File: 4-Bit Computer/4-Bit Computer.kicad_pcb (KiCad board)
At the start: 4 copper layers, 220.5 x 182.4 mm, 295 parts, among them J1 +12v, Q1 BC547, Q10 BC547, Q11 BC547, Q12 BC547, Q13 BC547, Q14 BC547, Q15 BC547, Q16 BC547, Q17 BC547, Q18 BC547, Q19 BC547, Q2 BC547, Q20 BC547, Q21 BC547, Q22 BC547, Q23 BC547, Q24 BC547, Q25 BC547, Q26 BC547, Q27 BC547, Q28 BC547, Q29 BC547, Q3 BC547, Q30 BC547, Q31 BC547, Q32 BC547, Q33 BC547, Q34 BC547, Q35 BC547, Q36 BC547, Q37 BC547, Q38 BC547, Q39 BC547, Q4 BC547, Q40 BC547, Q41 BC547, Q42 BC547, Q43 BC547, Q44 BC547, Q45 BC547, Q46 BC547, Q47 BC547, Q48 BC547, Q49 BC547, Q5 BC547, Q50 BC547, Q51 BC547, Q52 BC547, Q53 BC547, Q54 BC547, Q55 BC547, Q56 BC547, Q57 BC547, Q58 BC547, Q59 BC547, Q6 BC547, Q60 BC547, Q61 BC547, Q62 BC547, Q63 BC547, Q64 BC547, Q65 BC547, Q66 BC547, Q67 BC547, Q68 BC547, Q69 BC547, Q7 BC547, Q70 BC547, Q71 BC547, Q72 BC547, Q73 BC547, Q74 BC547, Q75 BC547, Q76 BC547, Q77 BC547, Q78 BC547, Q79 BC547, Q8 BC547, Q80 BC547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

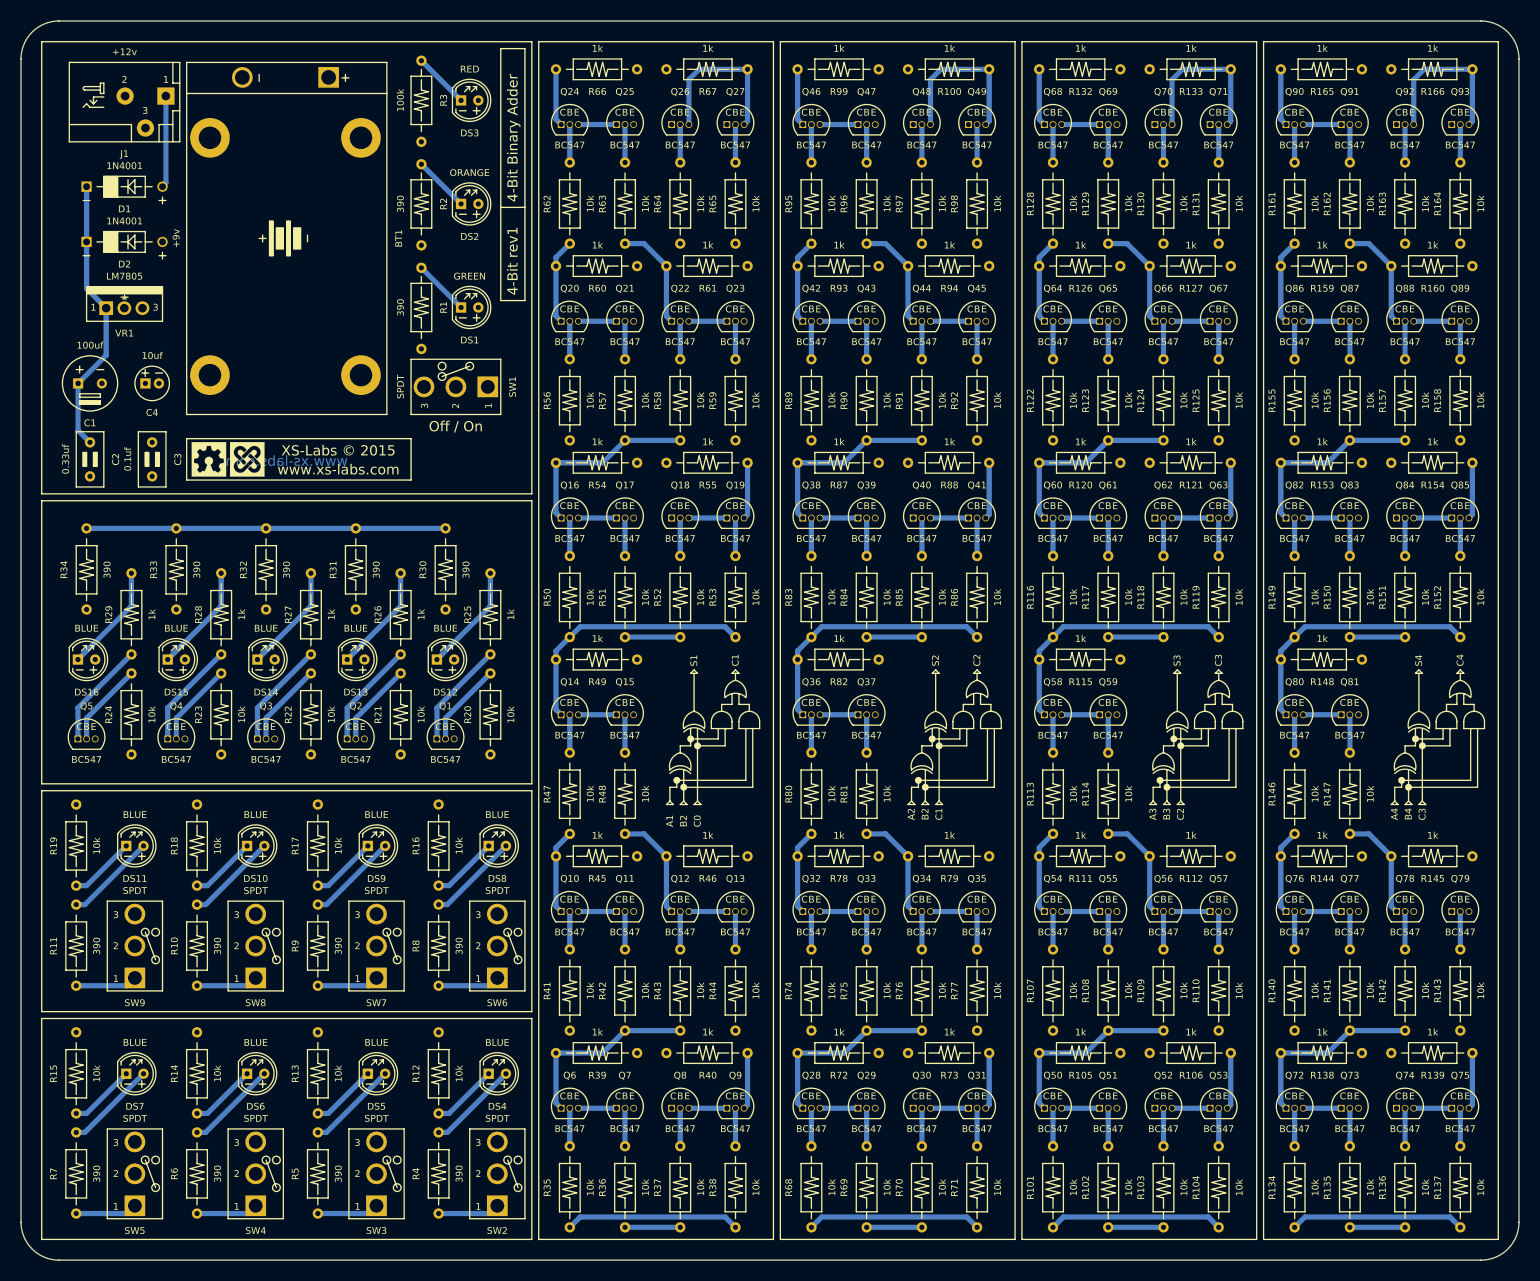
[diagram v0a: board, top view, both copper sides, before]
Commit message: Routing...
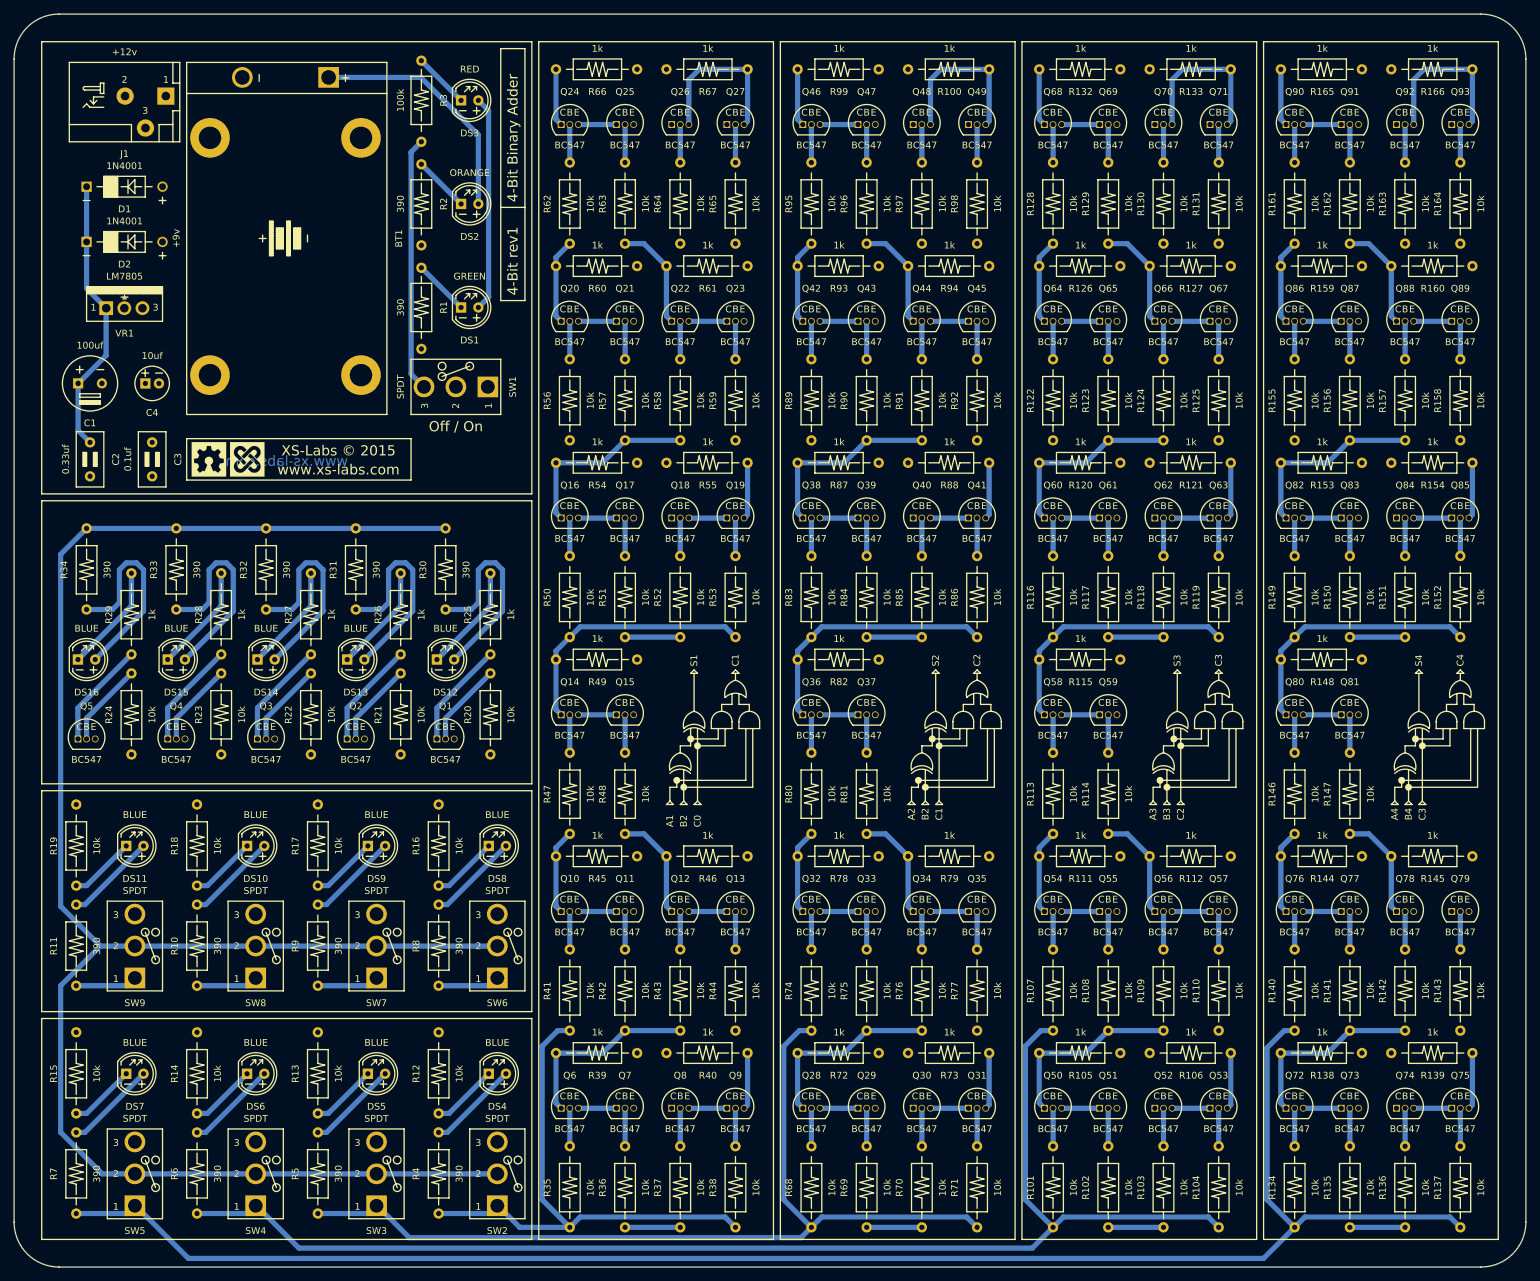
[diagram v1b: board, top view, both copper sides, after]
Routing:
- net Net-(R30-Pad1): track 52.8 -> 273.4 mm
- net A4: track 34.8 -> 243.8 mm
- net A3: track 34.8 -> 189.3 mm
- net A2: track 34.8 -> 134.7 mm
- net A1: track 34.8 -> 80.1 mm
- net Net-(R3-Pad1): track 0.00 -> 37.5 mm
- net Net-(BT1-Pad1): track 0.00 -> 35.7 mm
- net Net-(DS14-Pad2): track 0.00 -> 30.6 mm
- net Net-(DS16-Pad2): track 0.00 -> 30.6 mm
- net Net-(DS15-Pad2): track 0.00 -> 30.6 mm
- net Net-(DS12-Pad2): track 0.00 -> 30.6 mm
- net Net-(DS13-Pad2): track 0.00 -> 30.6 mm
- net Net-(D1-Pad2): track 13.5 -> 32.4 mm
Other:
- board size 220.5 x 182.4 mm -> 222.5 x 184.4 mm
